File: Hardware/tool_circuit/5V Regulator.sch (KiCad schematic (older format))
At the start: 14 parts, among them U1 TPS563211DRLR

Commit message: layout
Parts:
- removed C1: 22UF, KCM55QR7YA226KH01L:CAPC6153X390N, symbol KCM55QR7YA226KH01L:KCM55QR7YA226KH01L
- removed C2: 0.1UF, symbol CL31B104KBCNNNC:CL31B104KBCNNNC
- removed C3: 0.1UF, CL31B104KBCNNNC:CAPC3216X180N, symbol CL31B104KBCNNNC:CL31B104KBCNNNC
- removed C4: 10UF, 12063D106MAT2A:CAPC3216X178N, symbol 12063D106MAT2A:12063D106MAT2A
- removed D1: Green, WP7113GD:LED_WP7113GD, symbol WP7113GD:WP7113GD
- removed L1: 4.7UH, ul_SDR1307-4R7ML:SDR1307-4R7ML, symbol 2021-09-13_22-06-51:SDR1307-4R7ML
- removed R1: 820, CRGCQ1206F820R:RESC3115X65N, symbol CRGCQ1206F820R:CRGCQ1206F820R
- removed R2: 0, RK73Z2BTTD:RK73Z2BTTD, symbol 2021-10-08_20-10-06:RK73Z2BTTD
- removed R3: 10K, RNCP1206FTD10K0:RESC3115X60N, symbol RNCP1206FTD10K0:RNCP1206FTD10K0
- removed R4: 82K, ul_RC0603FR-0782KL:RC0603FR-0782KL, symbol 2021-09-13_22-27-50:RC0603FR-0782KL
- removed R5: 10K, CRCW040210K0DHEDP:RESC1005X40N, symbol CRCW040210K0DHEDP:CRCW040210K0DHEDP
- removed U1: TPS563211DRLR, ul_TPS563211DRLR:TPS563211DRLR, symbol TPS563211DRLR:TPS563211DRLR
- added C1: 100uF, EEUFS1K101:CAPPRD500W60D1000H1250, symbol EEUFS1K101:EEUFS1K101
- added C2: 1000uF, URS1E102MHD1TO:URS1E102MHD1TO, symbol 2021-10-30_20-57-30:URS1E102MHD1TO
- added CR1: B380-13-F, B380-13-F:B380-13-F, symbol 2021-10-30_21-29-43:B380-13-F
- added L1: 100 uH, IHLP-4040DZ_VIS:IHLP4040DZER101M11, symbol 2021-10-30_21-05-21:IHLP4040DZER101M11
- added U1: LM2576D2TR4-5G, LM2576D2TR4-5G:D2PAK-5, symbol LM2576D2TR4-5G:LM2576D2TR4-5G
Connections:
- net labels removed: 12V_LED
- wire segments 45 -> 19
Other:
- moved on the sheet: TP1, TP2

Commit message: layout
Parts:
- CR1: symbol 2021-10-30_21-29-43:B380-13-F -> tool_circuit-rescue:B380-13-F-2021-10-30_21-29-43
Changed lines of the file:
@@
 P 4050 3450
 F 0 "#PWR01" H 4050 3300 50  0001 C CNN
-F 1 "+12V" H 4065 3623 50  0000 C CNN
+F 1 "+12V" V 4150 3500 50  0000 C CNN
 F 2 "" H 4050 3450 50  0001 C CNN
 F 3 "" H 4050 3450 50  0001 C CNN
@@
 	4050 3450 4400 3450
 $Comp
-L 2021-10-30_21-29-43:B380-13-F CR1
+L tool_circuit-rescue:B380-13-F-2021-10-30_21-29-43 CR1
 U 1 1 6180A80C
 P 6350 3950
+AR Path="/6180A80C" Ref="CR1"  Part="1"
+AR Path="/611DBAE9/6131D12D/6180A80C" Ref="CR1"  Part="1"
 F 0 "CR1" V 6603 3846 60  0000 R CNN
 F 1 "B380-13-F" V 6497 3846 60  0000 R CNN

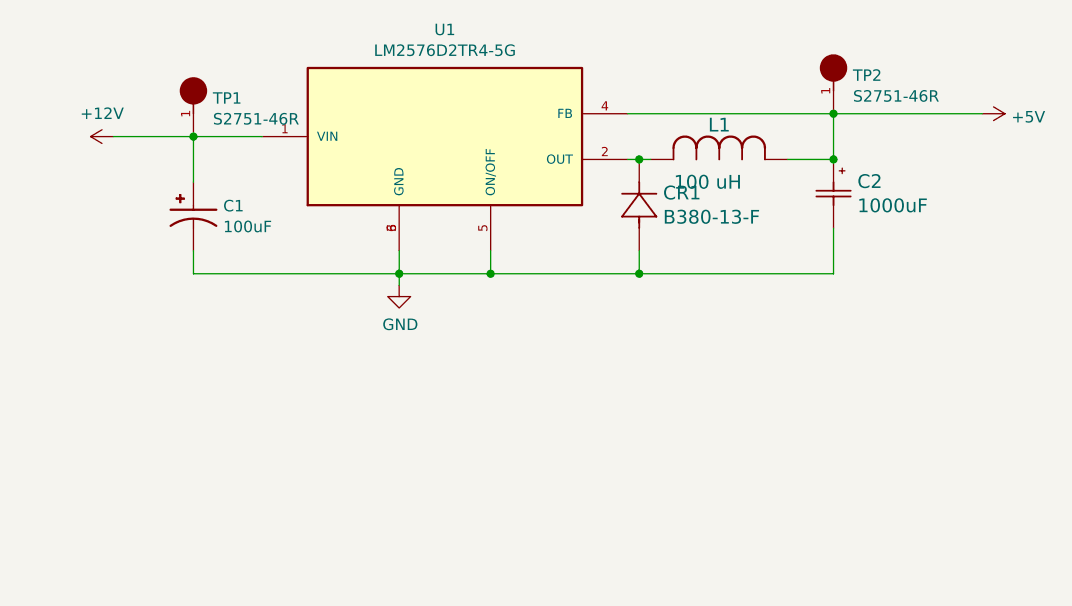
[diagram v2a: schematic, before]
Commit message: pcb revisions
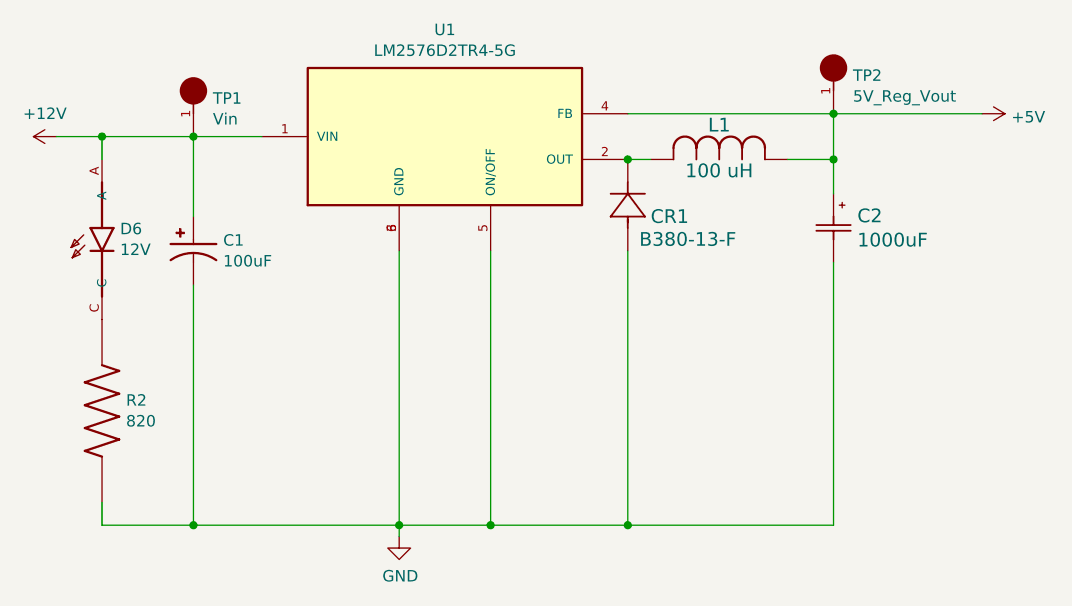
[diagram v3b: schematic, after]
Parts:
- added D6: 12V, WP7113GD:LED_WP7113GD, symbol WP7113GD:WP7113GD
- added R2: 820, CRGCQ1206F820R:RESC3115X65N, symbol CRGCQ1206F820R:CRGCQ1206F820R
- TP1: value S2751-46R -> Vin
- TP2: value S2751-46R -> 5V_Reg_Vout
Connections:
- net +12V: now also D6.A
- net GND: now also R2.2
- new net: D6.C, R2.1
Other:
- moved on the sheet: C1, C2, CR1
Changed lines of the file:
@@
 L power:+12V #PWR01
 U 1 1 614E38F8
-P 4050 3450
-F 0 "#PWR01" H 4050 3300 50  0001 C CNN
-F 1 "+12V" V 4150 3500 50  0000 C CNN
-F 2 "" H 4050 3450 50  0001 C CNN
-F 3 "" H 4050 3450 50  0001 C CNN
-	1    4050 3450
+P 3800 3450
+F 0 "#PWR01" H 3800 3300 50  0001 C CNN
+F 1 "+12V" V 3900 3500 50  0000 C CNN
+F 2 "" H 3800 3450 50  0001 C CNN
+F 3 "" H 3800 3450 50  0001 C CNN
+	1    3800 3450
 	0    -1   -1   0
 $EndComp
@@
 L power:GND #PWR02
 U 1 1 61401F04
-P 5300 4100
-F 0 "#PWR02" H 5300 3850 50  0001 C CNN
-F 1 "GND" H 5305 3927 50  0000 C CNN
-F 2 "" H 5300 4100 50  0001 C CNN
-F 3 "" H 5300 4100 50  0001 C CNN
-	1    5300 4100
+P 5300 5200
+F 0 "#PWR02" H 5300 4950 50  0001 C CNN
+F 1 "GND" H 5305 5027 50  0000 C CNN
+F 2 "" H 5300 5200 50  0001 C CNN
+F 3 "" H 5300 5200 50  0001 C CNN
+	1    5300 5200
 	1    0    0    -1
 $EndComp
@@
 P 4400 3350
 F 0 "TP1" H 4485 3417 50  0000 L CNN
-F 1 "S2751-46R" H 4485 3326 50  0000 L CNN
+F 1 "Vin" H 4485 3326 50  0000 L CNN
 F 2 "S2751-46R:HARWIN_S2751-46R" H 4400 3350 50  0001 L BNN
 F 3 "" H 4400 3350 50  0001 L BNN
@@
 	1    0    0    -1
 $EndComp
-Wire Wire Line
-	5300 3950 5300 4050
-Wire Wire Line
-	5700 3950 5700 4050
 $Comp
 L 2021-10-30_20-57-30:URS1E102MHD1TO C2
 U 1 1 617E34C7
-P 7200 3550
-F 0 "C2" V 7297 3654 60  0000 L CNN
-F 1 "1000uF" V 7403 3654 60  0000 L CNN
-F 2 "URS1E102MHD1TO:URS1E102MHD1TO" H 7350 3190 60  0001 C CNN
-F 3 "" H 7200 3550 60  0000 C CNN
-	1    7200 3550
-	0    1    1    0
-$EndComp
-Wire Wire Line
-	7200 3850 7200 4050
-Wire Wire Line
-	7200 4050 6350 4050
-Wire Wire Line
-	5700 4050 5300 4050
-Connection ~ 5700 4050
-Connection ~ 5300 4050
-Wire Wire Line
-	5300 4050 5300 4100
+P 7200 3700
+F 0 "C2" V 7297 3804 60  0000 L CNN
+F 1 "1000uF" V 7403 3804 60  0000 L CNN
+F 2 "URS1E102MHD1TO:URS1E102MHD1TO" H 7350 3340 60  0001 C CNN
+F 3 "" H 7200 3700 60  0000 C CNN
+	1    7200 3700
+	0    1    1    0
+$EndComp
+Wire Wire Line
+	5700 5150 5300 5150
+Connection ~ 5700 5150
+Connection ~ 5300 5150
+Wire Wire Line
+	5300 5150 5300 5200
 Wire Wire Line
 	6300 3350 7200 3350
@@
 P 7200 3250
 F 0 "TP2" H 7285 3317 50  0000 L CNN
-F 1 "S2751-46R" H 7285 3226 50  0000 L CNN
+F 1 "5V_Reg_Vout" H 7285 3226 50  0000 L CNN
 F 2 "S2751-46R:HARWIN_S2751-46R" H 7200 3250 50  0001 L BNN
 F 3 "" H 7200 3250 50  0001 L BNN
@@
 L EEUFS1K101:EEUFS1K101 C1
 U 1 1 617EC29C
-P 4400 3750
-F 0 "C1" V 4404 3880 50  0000 L CNN
-F 1 "100uF" V 4495 3880 50  0000 L CNN
-F 2 "EEUFS1K101:CAPPRD500W60D1000H1250" H 4400 3750 50  0001 L BNN
-F 3 "" H 4400 3750 50  0001 L BNN
-F 4 "28-FEB-20" H 4400 3750 50  0001 L BNN "PARTREV"
-F 5 "0.6" H 4400 3750 50  0001 L BNN "b_nom"
-F 6 "12.5" H 4400 3750 50  0001 L BNN "A_max"
-F 7 "10" H 4400 3750 50  0001 L BNN "D_nom"
-F 8 "0.65" H 4400 3750 50  0001 L BNN "b_max"
-F 9 "5" H 4400 3750 50  0001 L BNN "e_nom"
-F 10 "PANASONIC" H 4400 3750 50  0001 L BNN "MF"
-F 11 "FS-A" H 4400 3750 50  0001 L BNN "DESCRIPTION"
-	1    4400 3750
-	0    1    1    0
-$EndComp
-Wire Wire Line
-	4400 3650 4400 3450
+P 4400 3900
+F 0 "C1" V 4404 4030 50  0000 L CNN
+F 1 "100uF" V 4495 4030 50  0000 L CNN
+F 2 "EEUFS1K101:CAPPRD500W60D1000H1250" H 4400 3900 50  0001 L BNN
+F 3 "" H 4400 3900 50  0001 L BNN
+F 4 "28-FEB-20" H 4400 3900 50  0001 L BNN "PARTREV"
+F 5 "0.6" H 4400 3900 50  0001 L BNN "b_nom"
+F 6 "12.5" H 4400 3900 50  0001 L BNN "A_max"
+F 7 "10" H 4400 3900 50  0001 L BNN "D_nom"
+F 8 "0.65" H 4400 3900 50  0001 L BNN "b_max"
+F 9 "5" H 4400 3900 50  0001 L BNN "e_nom"
+F 10 "PANASONIC" H 4400 3900 50  0001 L BNN "MF"
+F 11 "FS-A" H 4400 3900 50  0001 L BNN "DESCRIPTION"
+	1    4400 3900
+	0    1    1    0
+$EndComp
 Connection ~ 4400 3450
 Wire Wire Line
 	4400 3450 4700 3450
-Wire Wire Line
-	4400 3950 4400 4050
-Wire Wire Line
-	4400 4050 5300 4050
 $Comp
 L 2021-10-30_21-05-21:IHLP4040DZER101M11 L1
@@
 P 6400 3550
 F 0 "L1" H 6700 3700 60  0000 C CNN
-F 1 "100 uH" H 6650 3450 60  0000 C CNN
+F 1 "100 uH" H 6700 3500 60  0000 C CNN
 F 2 "IHLP-4040DZ_VIS:IHLP4040DZER101M11" H 6675 3265 60  0001 C CNN
 F 3 "" H 6400 3550 60  0000 C CNN
@@
 $EndComp
 Wire Wire Line
-	6300 3550 6350 3550
-Wire Wire Line
 	7000 3550 7200 3550
+$Comp
+L tool_circuit-rescue:B380-13-F-2021-10-30_21-29-43 CR?
+U 1 1 6180A80C
+P 6300 3950
+AR Path="/6180A80C" Ref="CR?"  Part="1"
+AR Path="/611DBAE9/6131D12D/6180A80C" Ref="CR1"  Part="1"
+F 0 "CR1" V 6450 3850 60  0000 R CNN
+F 1 "B380-13-F" V 6350 3900 60  0000 R CNN
+F 2 "B380-13-F:B380-13-F" H 6500 3590 60  0001 C CNN
+F 3 "" H 6300 3950 60  0000 C CNN
+	1    6300 3950
+	0    -1   -1   0
+$EndComp
+$Comp
+L CRGCQ1206F820R:CRGCQ1206F820R R2
+U 1 1 61883CC7
+P 4000 4650
+F 0 "R2" V 3954 4755 50  0000 L CNN
+F 1 "820" V 4045 4755 50  0000 L CNN
+F 2 "CRGCQ1206F820R:RESC3115X65N" H 4000 4650 50  0001 L BNN
+F 3 "" H 4000 4650 50  0001 L BNN
+F 4 "2-2176343-4" H 4000 4650 50  0001 L BNN "Comment"
+	1    4000 4650
+	0    1    1    0
+$EndComp
+Wire Wire Line
+	4400 4100 4400 5150
+Wire Wire Line
+	4400 5150 5300 5150
+Wire Wire Line
+	7200 4000 7200 5150
+$Comp
+L WP7113GD:WP7113GD D6
+U 1 1 61894810
+P 4000 3950
+F 0 "D6" V 4096 3871 50  0000 R CNN
+F 1 "12V" V 4005 3871 50  0000 R CNN
+F 2 "WP7113GD:LED_WP7113GD" H 4000 3950 50  0001 L BNN
+F 3 "" H 4000 3950 50  0001 L BNN
+F 4 "Kingbright" H 4000 3950 50  0001 L BNN "MANUFACTURER"
+	1    4000 3950
+	0    -1   -1   0
+$EndComp
+Wire Wire Line
+	3800 3450 4000 3450
+Wire Wire Line
+	4000 3450 4000 3550
+Connection ~ 4000 3450
+Wire Wire Line
+	4000 3450 4400 3450
+Wire Wire Line
+	4000 5050 4000 5150
+Wire Wire Line
+	4000 5150 4400 5150
+Connection ~ 4400 5150
+Wire Wire Line
+	4400 3450 4400 3800
+Wire Wire Line
+	5300 3950 5300 5150
+Wire Wire Line
+	5700 3950 5700 5150
+Wire Wire Line
+	5700 5150 6300 5150
+Wire Wire Line
+	6300 3550 6400 3550
+Connection ~ 6300 3550
+Wire Wire Line
+	6300 3950 6300 5150
+Connection ~ 6300 5150
+Wire Wire Line
+	6300 5150 7200 5150
+Wire Wire Line
+	7200 3700 7200 3550
 Connection ~ 7200 3550
-Wire Wire Line
-	4050 3450 4400 3450
-$Comp
-L tool_circuit-rescue:B380-13-F-2021-10-30_21-29-43 CR1
-U 1 1 6180A80C
-P 6350 3950
-AR Path="/6180A80C" Ref="CR1"  Part="1"
-AR Path="/611DBAE9/6131D12D/6180A80C" Ref="CR1"  Part="1"
-F 0 "CR1" V 6603 3846 60  0000 R CNN
-F 1 "B380-13-F" V 6497 3846 60  0000 R CNN
-F 2 "B380-13-F:B380-13-F" H 6550 3590 60  0001 C CNN
-F 3 "" H 6350 3950 60  0000 C CNN
-	1    6350 3950
-	0    -1   -1   0
-$EndComp
-Connection ~ 6350 3550
-Wire Wire Line
-	6350 3550 6400 3550
-Wire Wire Line
-	6350 3950 6350 4050
-Connection ~ 6350 4050
-Wire Wire Line
-	6350 4050 5700 4050
 $EndSCHEMATC

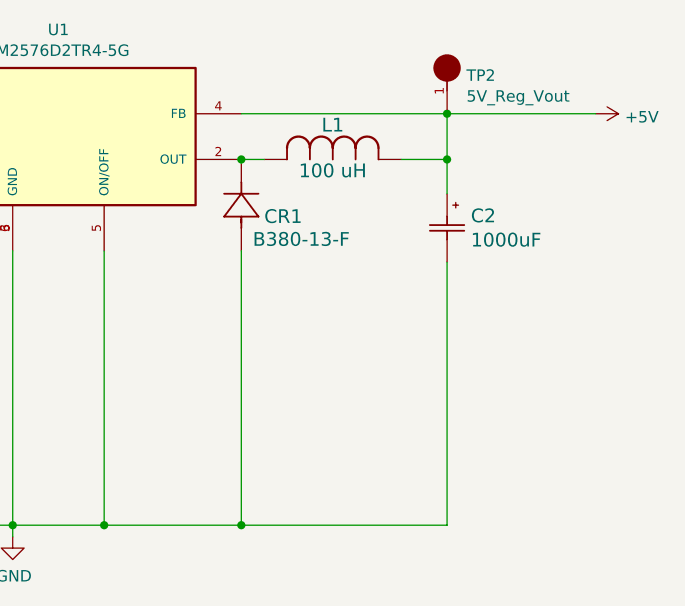
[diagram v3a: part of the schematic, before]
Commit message: pcb
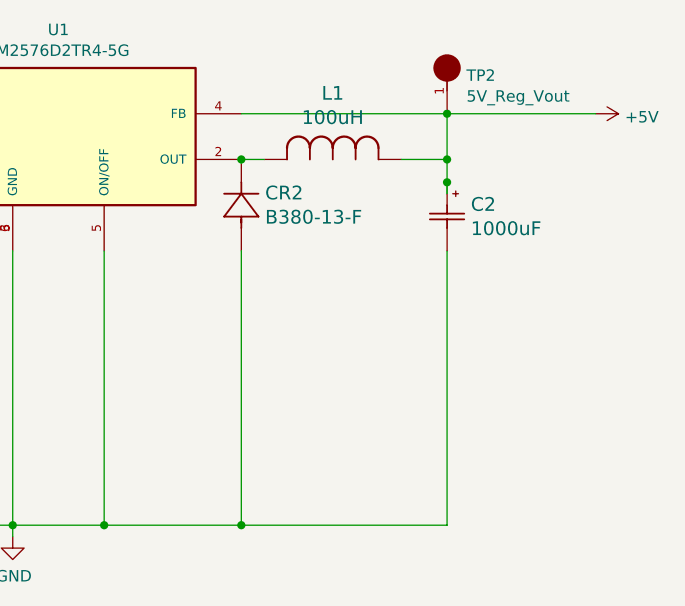
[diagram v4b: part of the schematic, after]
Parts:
- removed CR1: B380-13-F, B380-13-F:B380-13-F, symbol tool_circuit-rescue:B380-13-F-2021-10-30_21-29-43
- added CR2: B380-13-F, B380-13-F:B380-13-F, symbol 2021-10-30_21-29-43:B380-13-F
- L1: value 100 uH -> 100uH
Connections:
- wire segments 23 -> 24
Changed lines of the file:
@@
 	1    0    0    -1
-$EndComp
-$Comp
-L 2021-10-30_20-57-30:URS1E102MHD1TO C2
-U 1 1 617E34C7
-P 7200 3700
-F 0 "C2" V 7297 3804 60  0000 L CNN
-F 1 "1000uF" V 7403 3804 60  0000 L CNN
-F 2 "URS1E102MHD1TO:URS1E102MHD1TO" H 7350 3340 60  0001 C CNN
-F 3 "" H 7200 3700 60  0000 C CNN
-	1    7200 3700
-	0    1    1    0
 $EndComp
 Wire Wire Line
@@
 Wire Wire Line
 	4400 3450 4700 3450
-$Comp
-L 2021-10-30_21-05-21:IHLP4040DZER101M11 L1
-U 1 1 617F1E2E
-P 6400 3550
-F 0 "L1" H 6700 3700 60  0000 C CNN
-F 1 "100 uH" H 6700 3500 60  0000 C CNN
-F 2 "IHLP-4040DZ_VIS:IHLP4040DZER101M11" H 6675 3265 60  0001 C CNN
-F 3 "" H 6400 3550 60  0000 C CNN
-	1    6400 3550
-	1    0    0    -1
-$EndComp
 Wire Wire Line
 	7000 3550 7200 3550
-$Comp
-L tool_circuit-rescue:B380-13-F-2021-10-30_21-29-43 CR?
-U 1 1 6180A80C
-P 6300 3950
-AR Path="/6180A80C" Ref="CR?"  Part="1"
-AR Path="/611DBAE9/6131D12D/6180A80C" Ref="CR1"  Part="1"
-F 0 "CR1" V 6450 3850 60  0000 R CNN
-F 1 "B380-13-F" V 6350 3900 60  0000 R CNN
-F 2 "B380-13-F:B380-13-F" H 6500 3590 60  0001 C CNN
-F 3 "" H 6300 3950 60  0000 C CNN
-	1    6300 3950
-	0    -1   -1   0
-$EndComp
 $Comp
 L CRGCQ1206F820R:CRGCQ1206F820R R2
@@
 Wire Wire Line
 	4400 5150 5300 5150
-Wire Wire Line
-	7200 4000 7200 5150
 $Comp
 L WP7113GD:WP7113GD D6
@@
 	6300 5150 7200 5150
 Wire Wire Line
-	7200 3700 7200 3550
+	7200 3700 7200 3650
 Connection ~ 7200 3550
+Connection ~ 7200 3650
+Wire Wire Line
+	7200 3650 7200 3550
+Wire Wire Line
+	7200 3950 7200 5150
+$Comp
+L 2021-10-30_20-57-30:URS1E102MHD1TO C2
+U 1 1 61A5367C
+P 7200 3650
+F 0 "C2" V 7297 3754 60  0000 L CNN
+F 1 "1000uF" V 7403 3754 60  0000 L CNN
+F 2 "URS1E102MHD1TO:URS1E102MHD1TO" H 7350 3290 60  0001 C CNN
+F 3 "" H 7200 3650 60  0000 C CNN
+	1    7200 3650
+	0    1    1    0
+$EndComp
+$Comp
+L 2021-10-30_21-29-43:B380-13-F CR2
+U 1 1 61A8BA56
+P 6300 3950
+F 0 "CR2" V 6553 3846 60  0000 R CNN
+F 1 "B380-13-F" V 6447 3846 60  0000 R CNN
+F 2 "B380-13-F:B380-13-F" H 6500 3590 60  0001 C CNN
+F 3 "" H 6300 3950 60  0000 C CNN
+	1    6300 3950
+	0    -1   -1   0
+$EndComp
+$Comp
+L 2021-10-30_21-05-21:IHLP4040DZER101M11 L1
+U 1 1 61A8D233
+P 6400 3550
+F 0 "L1" H 6700 3839 60  0000 C CNN
+F 1 "100uH" H 6700 3733 60  0000 C CNN
+F 2 "IHLP-4040DZ_VIS:IHLP4040DZER101M11" H 6675 3265 60  0001 C CNN
+F 3 "" H 6400 3550 60  0000 C CNN
+	1    6400 3550
+	1    0    0    -1
+$EndComp
 $EndSCHEMATC
